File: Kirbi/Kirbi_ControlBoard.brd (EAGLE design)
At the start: 66 x 56 mm, 73 parts, among them J1 JST_PH_1X03_90, J10 JST_PH_1X03, J11 TE_02X01_3.96MM, J12 MOLEX_1.25MM_4PIN_90, J15 JST_PH_1X03_90, J2 JST_PH_1X03_90, J3 MOLEX_1.25MM_4PIN_90, J4 MOLEX_1.25MM_4PIN_90, J5 JST_PH_1X03_90, J6 JST_PH_1X03_90, J7 JST_PH_1X03_90, J8 JST_PH_1X03_90, J9 JST_PH_1X03, U1 TEENSY_3.6_DIL, U2 AP2114H-3.3TRG1, U3 AP2114H-1.8TRG1, U4 ICM-20948, U5 LM339-14-SOIC

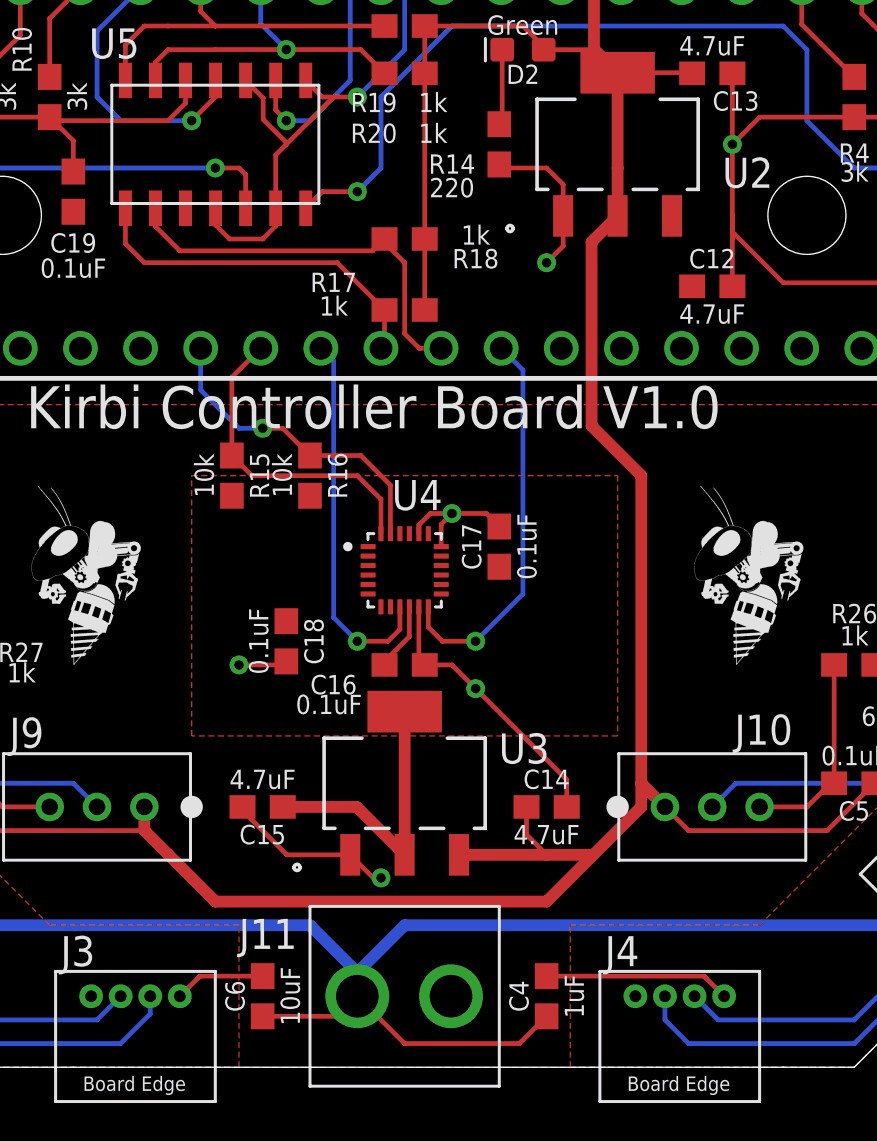
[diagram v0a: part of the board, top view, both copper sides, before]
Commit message: level shifter
added level shifter to gucci and kirbi. the part is in gucci's library. the relevant area on the boards should be very similar, but not identical
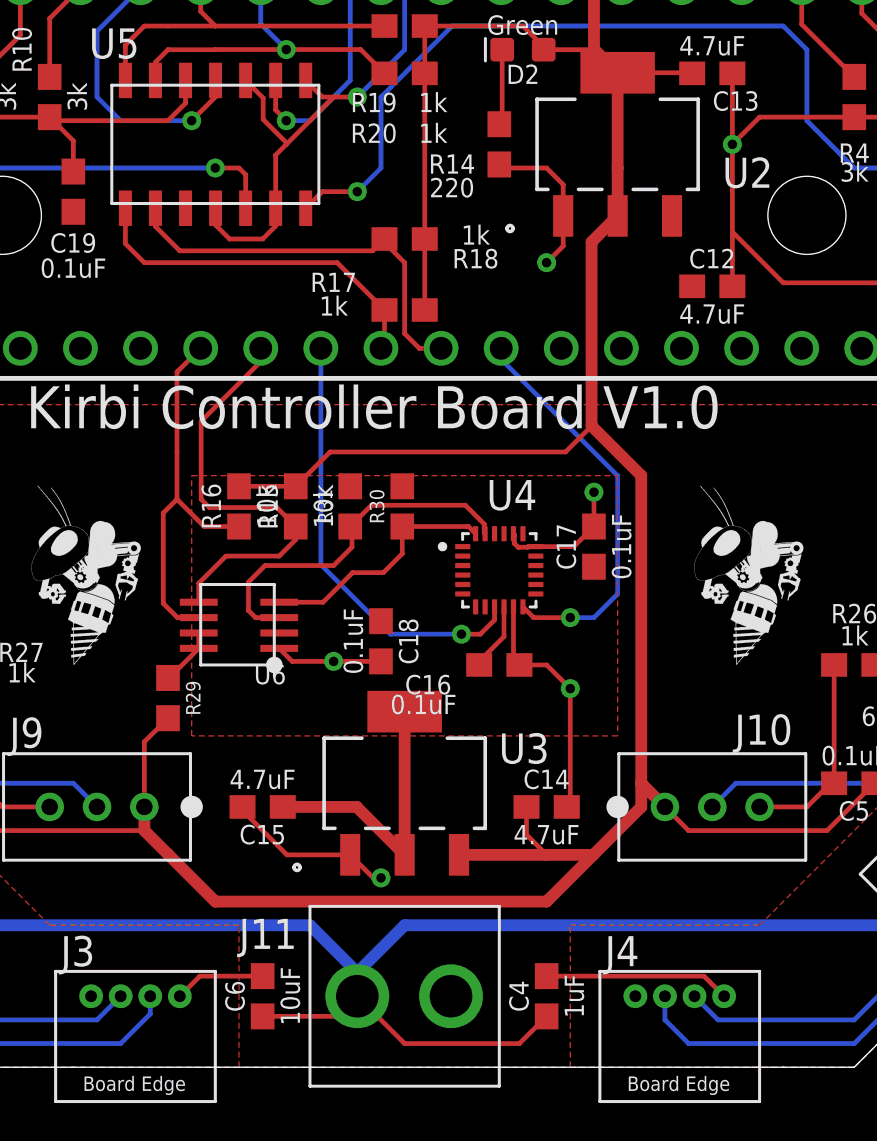
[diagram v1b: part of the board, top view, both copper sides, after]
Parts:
- added R29: 200k, SparkFun-Resistors:0603
- added R30, R31: 10k, SparkFun-Resistors:0603
- added U6: PCA9306_LSSOP, Gucci_ControlBoard:8-LSSOP
- moved C16 4.00 mm to (23.0, 17.0)
- moved C17 4.00 mm to (27.0, 22.0)
- moved C18 4.00 mm to (18.0, 18.0)
- moved U4 4.00 mm to (23.0, 21.0)
- moved R16 3.27 mm to (12.0, 23.7), turned to 90 degrees
- moved R15 3.00 mm to (14.4, 23.7), turned to 90 degrees
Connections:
- new net N$4: R29.1, U6.P$7, U6.P$8
- new net SCL2: R16.1, U1.7, U6.P$6
- new net SDA2: R15.1, U1.8, U6.P$5
- net 1.8V: now also R30.2, R31.2, U6.P$2; no longer R15.2, R16.2
- net 3V3: now also R15.2, R16.2, R29.2
- net GND: now also U6.P$1
- net SCL1: now also R31.1, U6.P$3; no longer R16.1, U1.7
- net SDA1: now also R30.1, U6.P$4; no longer R15.1, U1.8
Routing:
- net 3V3: track 152.7 -> 172.8 mm
- net SDA2: track 0.00 -> 18.1 mm
- net SCL2: track 0.00 -> 16.3 mm
- net SDA1: track 13.6 -> 10.4 mm
- net IMU_AD0: track 16.0 -> 18.5 mm
- net N$4: track 0.00 -> 2.47 mm
- net SCL1: track 13.5 -> 15.3 mm, vias 1 -> 0
